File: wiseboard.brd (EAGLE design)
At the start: 87 x 67 mm, 85 parts, among them IC2 LM358MX, Q1 IRLML6402TRPBF, Q2 IRLML6402TRPBF, U1 LT1945EMSPBF, U2 BQ24210DQCT, X1 1528-1438-ND

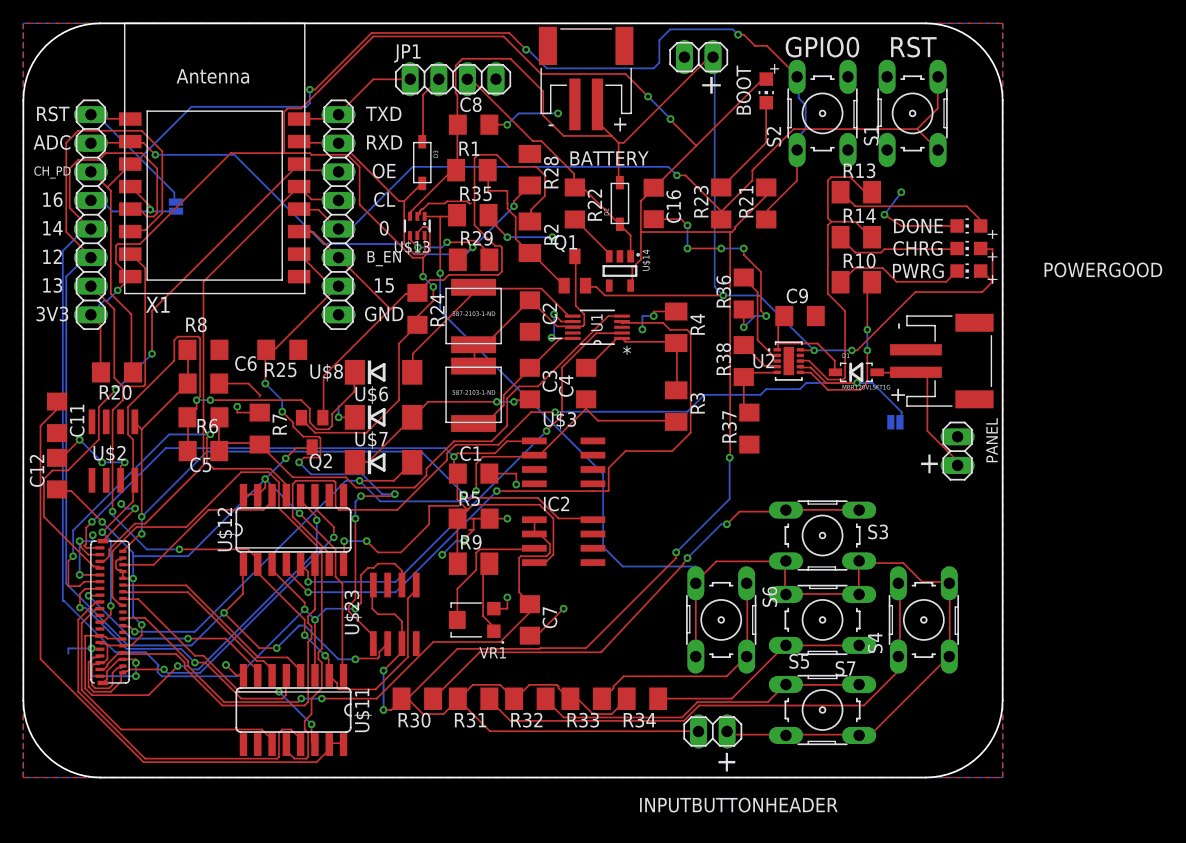
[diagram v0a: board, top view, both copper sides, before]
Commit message: FINAL REV1.5 PCB LAYOUT
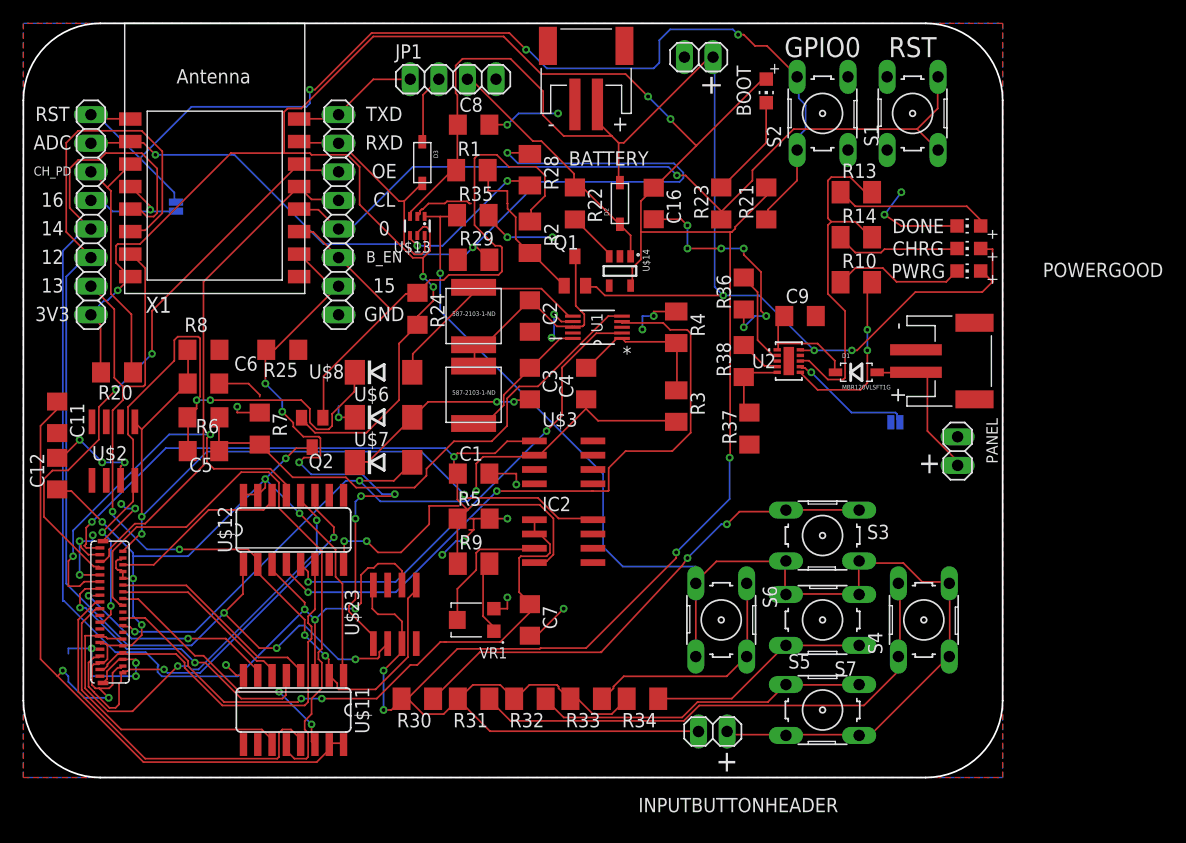
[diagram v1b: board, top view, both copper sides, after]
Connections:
- removed net N$16: C11.1, U$11.15, U$11.16
- removed net N$24: R29.2, U$13.4
- new net N$12: R28.2, U$13.4
- net ADC: now also R28.1, R29.2; no longer R28.2, R29.1
- net CHARGE_EN: no longer U$12.7
- net GND: now also R29.1; no longer R28.1
- net VDD: now also C11.1, U$11.15, U$11.16
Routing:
- net CHARGE_EN: track 78.7 -> 11.2 mm, vias 2 -> 1
- net VDD: track 76.8 -> 139.3 mm, vias 6 -> 8
- net N$16: track 55.3 -> 0.00 mm
- net ADC: track 47.8 -> 80.5 mm
- net N$12: track 0.00 -> 14.0 mm, vias 0 -> 2
- net N$24: track 8.99 -> 0.00 mm, vias 2 -> 0
- net QP7@2: track 36.4 -> 38.6 mm
- net QP6@2: track 40.5 -> 41.7 mm
